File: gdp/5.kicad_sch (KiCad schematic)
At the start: 10 parts, among them IC29 74LS538, IC30 74LS538, IC67 74LS166, IC68 74LS30, IC69 74LS166, IC70 74LS30

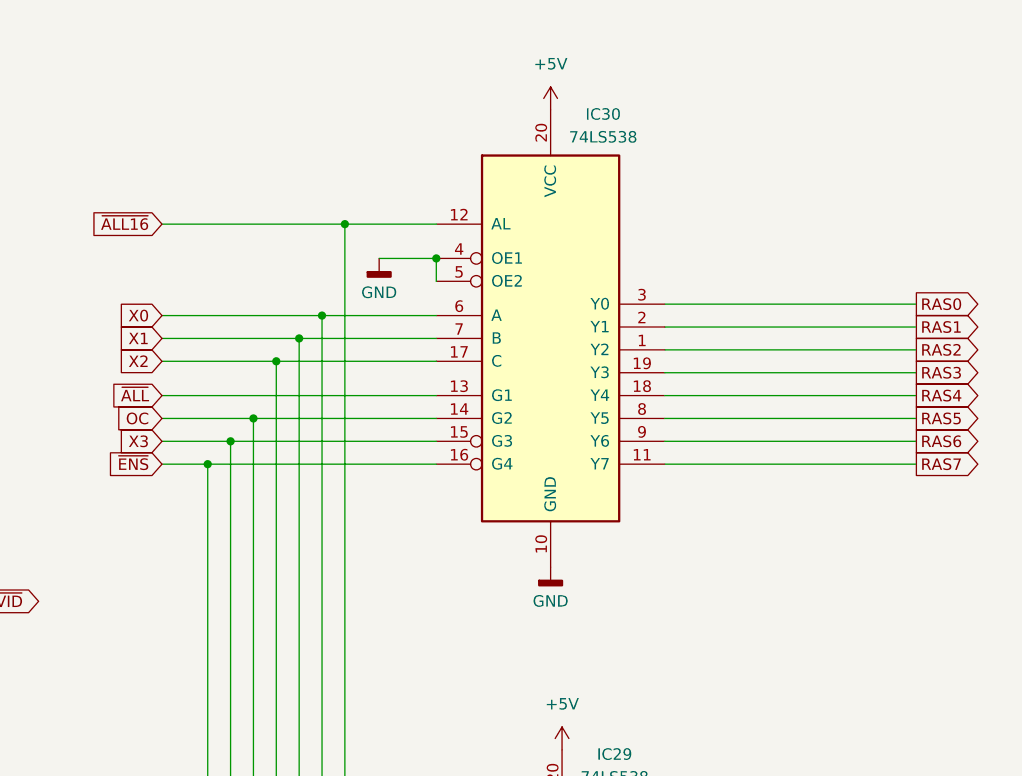
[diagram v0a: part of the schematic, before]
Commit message: Adds Sheet 12
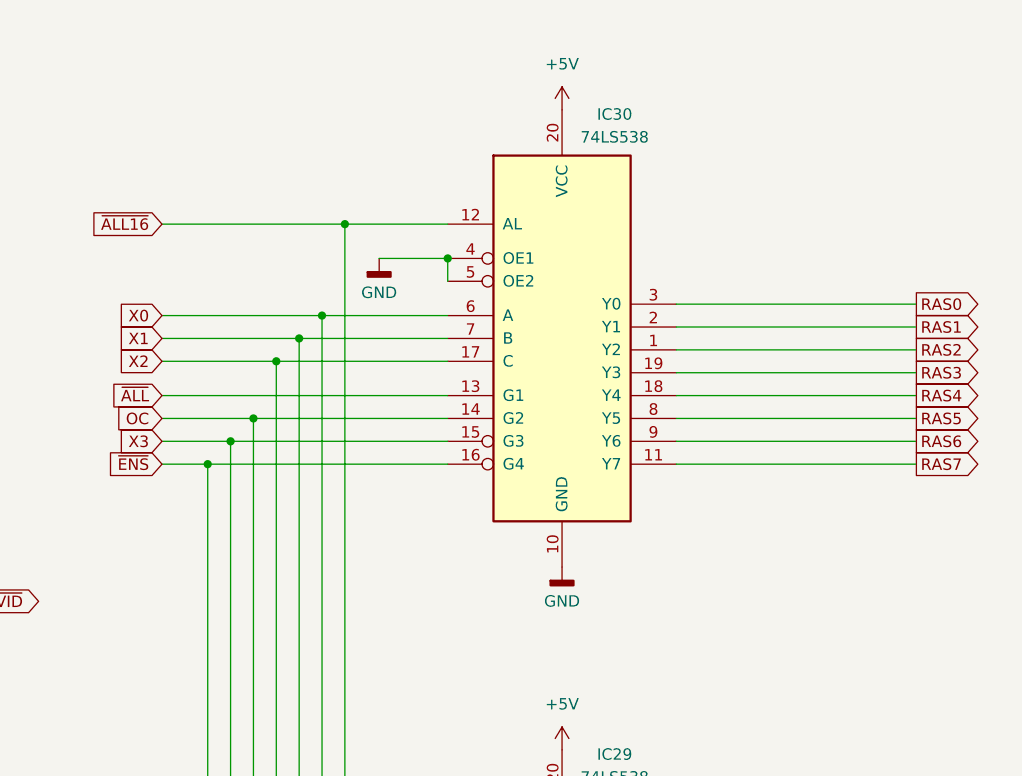
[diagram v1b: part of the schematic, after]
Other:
- moved on the sheet: IC30
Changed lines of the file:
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@@
 	)
 	(junction
-		(at 208.28 46.99)
+		(at 209.55 46.99)
 		(diameter 0)
 		(color 0 0 0 0)
@@
 	(wire
 		(pts
-			(xy 190.5 58.42) (xy 208.28 58.42)
+			(xy 190.5 58.42) (xy 209.55 58.42)
 		)
 		(stroke
@@
 	(wire
 		(pts
-			(xy 187.96 64.77) (xy 208.28 64.77)
+			(xy 187.96 64.77) (xy 209.55 64.77)
 		)
 		(stroke
@@
 	(wire
 		(pts
-			(xy 193.04 55.88) (xy 208.28 55.88)
+			(xy 193.04 55.88) (xy 209.55 55.88)
 		)
 		(stroke
@@
 	(wire
 		(pts
-			(xy 233.68 52.07) (xy 261.62 52.07)
+			(xy 234.95 52.07) (xy 261.62 52.07)
 		)
 		(stroke
@@
 	(wire
 		(pts
-			(xy 201.93 46.99) (xy 208.28 46.99)
+			(xy 201.93 46.99) (xy 209.55 46.99)
 		)
 		(stroke
@@
 	(wire
 		(pts
-			(xy 233.68 57.15) (xy 261.62 57.15)
+			(xy 234.95 57.15) (xy 261.62 57.15)
 		)
 		(stroke
@@
 	(wire
 		(pts
-			(xy 233.68 64.77) (xy 261.62 64.77)
+			(xy 234.95 64.77) (xy 261.62 64.77)
 		)
 		(stroke
@@
 	(wire
 		(pts
-			(xy 233.68 69.85) (xy 261.62 69.85)
+			(xy 234.95 69.85) (xy 261.62 69.85)
 		)
 		(stroke
@@
 	(wire
 		(pts
-			(xy 233.68 62.23) (xy 261.62 62.23)
+			(xy 234.95 62.23) (xy 261.62 62.23)
 		)
 		(stroke
@@
 	(wire
 		(pts
-			(xy 233.68 59.69) (xy 261.62 59.69)
+			(xy 234.95 59.69) (xy 261.62 59.69)
 		)
 		(stroke
@@
 	(wire
 		(pts
-			(xy 198.12 43.18) (xy 208.28 43.18)
+			(xy 198.12 43.18) (xy 209.55 43.18)
 		)
 		(stroke
@@
 	(wire
 		(pts
-			(xy 177.8 62.23) (xy 208.28 62.23)
+			(xy 177.8 62.23) (xy 209.55 62.23)
 		)
 		(stroke
@@
 	(wire
 		(pts
-			(xy 195.58 53.34) (xy 208.28 53.34)
+			(xy 195.58 53.34) (xy 209.55 53.34)
 		)
 		(stroke
@@
 	(wire
 		(pts
-			(xy 233.68 54.61) (xy 261.62 54.61)
+			(xy 234.95 54.61) (xy 261.62 54.61)
 		)
 		(stroke
@@
 	(wire
 		(pts
-			(xy 208.28 46.99) (xy 208.28 49.53)
+			(xy 234.95 67.31) (xy 261.62 67.31)
 		)
 		(stroke
@@
 	(wire
 		(pts
-			(xy 233.68 67.31) (xy 261.62 67.31)
+			(xy 110.49 55.88) (xy 115.57 55.88)
 		)
 		(stroke
@@
 	(wire
 		(pts
-			(xy 110.49 55.88) (xy 115.57 55.88)
+			(xy 209.55 46.99) (xy 209.55 49.53)
 		)
 		(stroke
@@
 	(wire
 		(pts
-			(xy 182.88 69.85) (xy 208.28 69.85)
+			(xy 182.88 69.85) (xy 209.55 69.85)
 		)
 		(stroke
@@
 	(wire
 		(pts
-			(xy 185.42 67.31) (xy 208.28 67.31)
+			(xy 185.42 67.31) (xy 209.55 67.31)
 		)
 		(stroke
@@
 	(symbol
 		(lib_id "power:GNDD")
-		(at 220.98 81.28 0)
+		(at 222.25 81.28 0)
 		(unit 1)
 		(exclude_from_sim no)
@@
 		(fields_autoplaced yes)
 		(property "Reference" "#PWR095"
-			(at 220.98 87.63 0)
+			(at 222.25 87.63 0)
 			(effects
 				(font
@@
 		)
 		(property "Value" "GND"
-			(at 220.98 85.09 0)
+			(at 222.25 85.09 0)
 			(effects
 				(font
@@
 		)
 		(property "Footprint" ""
-			(at 220.98 81.28 0)
+			(at 222.25 81.28 0)
 			(effects
 				(font
@@
 		)
 		(property "Datasheet" ""
-			(at 220.98 81.28 0)
+			(at 222.25 81.28 0)
 			(effects
 				(font
@@
 		)
 		(property "Description" "Power symbol creates a global label with name \"GNDD\" , digital ground"
-			(at 220.98 81.28 0)
+			(at 222.25 81.28 0)
 			(effects
 				(font
@@
 	(symbol
 		(lib_id "power:+5V")
-		(at 220.98 30.48 0)
+		(at 222.25 30.48 0)
 		(unit 1)
 		(exclude_from_sim no)
@@
 		(fields_autoplaced yes)
 		(property "Reference" "#PWR094"
-			(at 220.98 34.29 0)
+			(at 222.25 34.29 0)
 			(effects
 				(font
@@
 		)
 		(property "Value" "+5V"
-			(at 220.98 25.4 0)
+			(at 222.25 25.4 0)
 			(effects
 				(font
@@
 		)
 		(property "Footprint" ""
-			(at 220.98 30.48 0)
+			(at 222.25 30.48 0)
 			(effects
 				(font
@@
 		)
 		(property "Datasheet" ""
-			(at 220.98 30.48 0)
+			(at 222.25 30.48 0)
 			(effects
 				(font
@@
 		)
 		(property "Description" "Power symbol creates a global label with name \"+5V\""
-			(at 220.98 30.48 0)
+			(at 222.25 30.48 0)
 			(effects
 				(font
@@
 		(lib_name "74LS166_1")
 		(lib_id "74xx:74LS166")
-		(at 220.98 55.88 0)
+		(at 222.25 55.88 0)
 		(unit 1)
 		(exclude_from_sim no)
@@
 		(fields_autoplaced yes)
 		(property "Reference" "IC30"
-			(at 226.822 30.988 0)
+			(at 228.092 30.988 0)
 			(do_not_autoplace yes)
 			(effects
@@
 		)
 		(property "Value" "74LS538"
-			(at 226.822 33.528 0)
+			(at 228.092 33.528 0)
 			(do_not_autoplace yes)
 			(effects
@@
 		)
 		(property "Footprint" ""
-			(at 220.98 55.88 0)
+			(at 222.25 55.88 0)
 			(effects
 				(font
@@
 		)
 		(property "Datasheet" "N/A"
-			(at 180.34 53.848 0)
+			(at 181.61 53.848 0)
 			(effects
 				(font
@@
 		)
 		(property "Description" "Decoder"
-			(at 180.34 50.292 0)
+			(at 181.61 50.292 0)
 			(effects
 				(font
